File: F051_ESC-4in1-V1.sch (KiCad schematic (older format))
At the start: 39 parts, among them J1 Conn_01x02, J11 Conn_01x03, J14 Conn_01x03, J2 Conn_01x10, J3 Conn_01x05, J4 Conn_01x05, J5 Conn_01x05, J6 Conn_01x03, J7 Conn_01x05, J8 Conn_01x03, J9 Conn_01x10

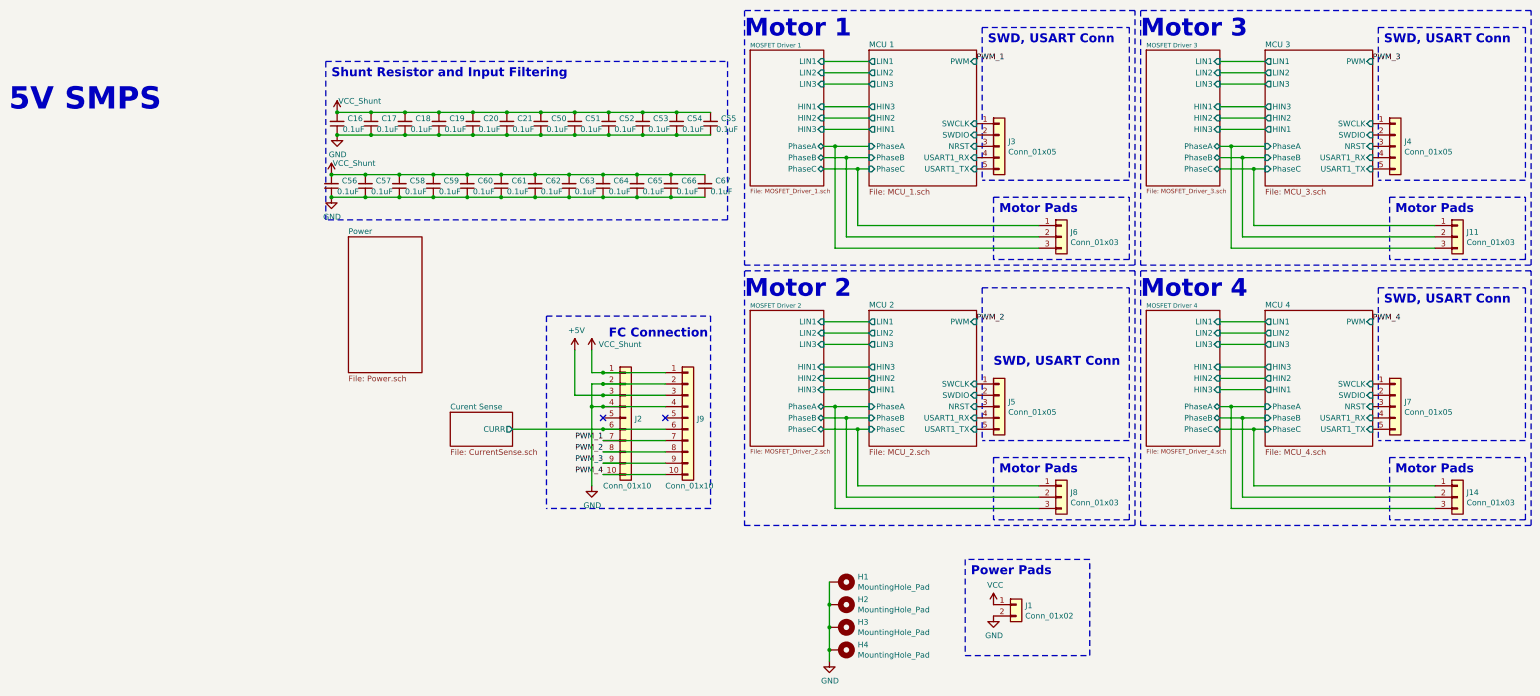
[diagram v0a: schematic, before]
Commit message: Added more PNGs
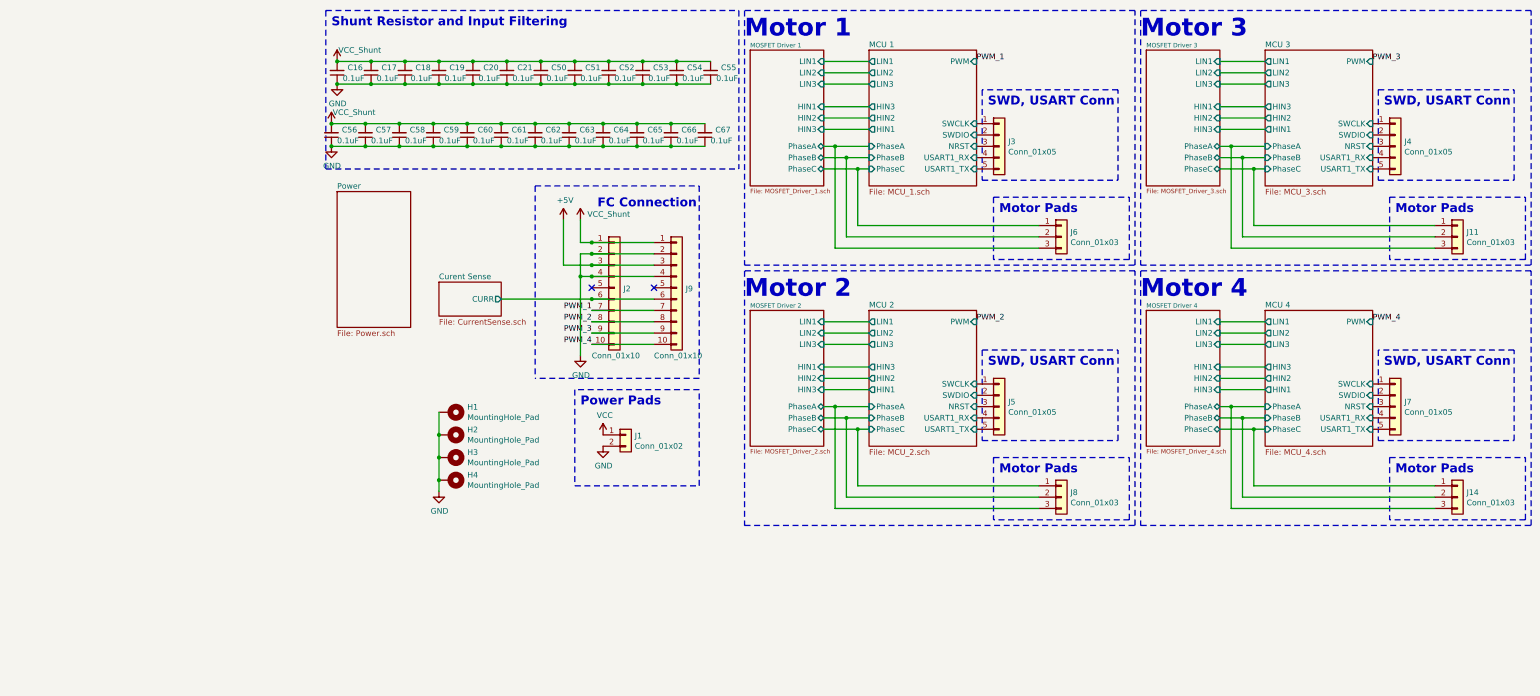
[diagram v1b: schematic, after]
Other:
- note removed: "5V SMPS"
- moved on the sheet: C16, C17, C18, C19, C20, C21, C50, C51, C52, C53, C54, C55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
